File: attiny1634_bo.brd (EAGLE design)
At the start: 49.5 x 22.2 mm, 11 parts, among them J1 AVR_SPI_PRG_6NS, Y1 12MHz

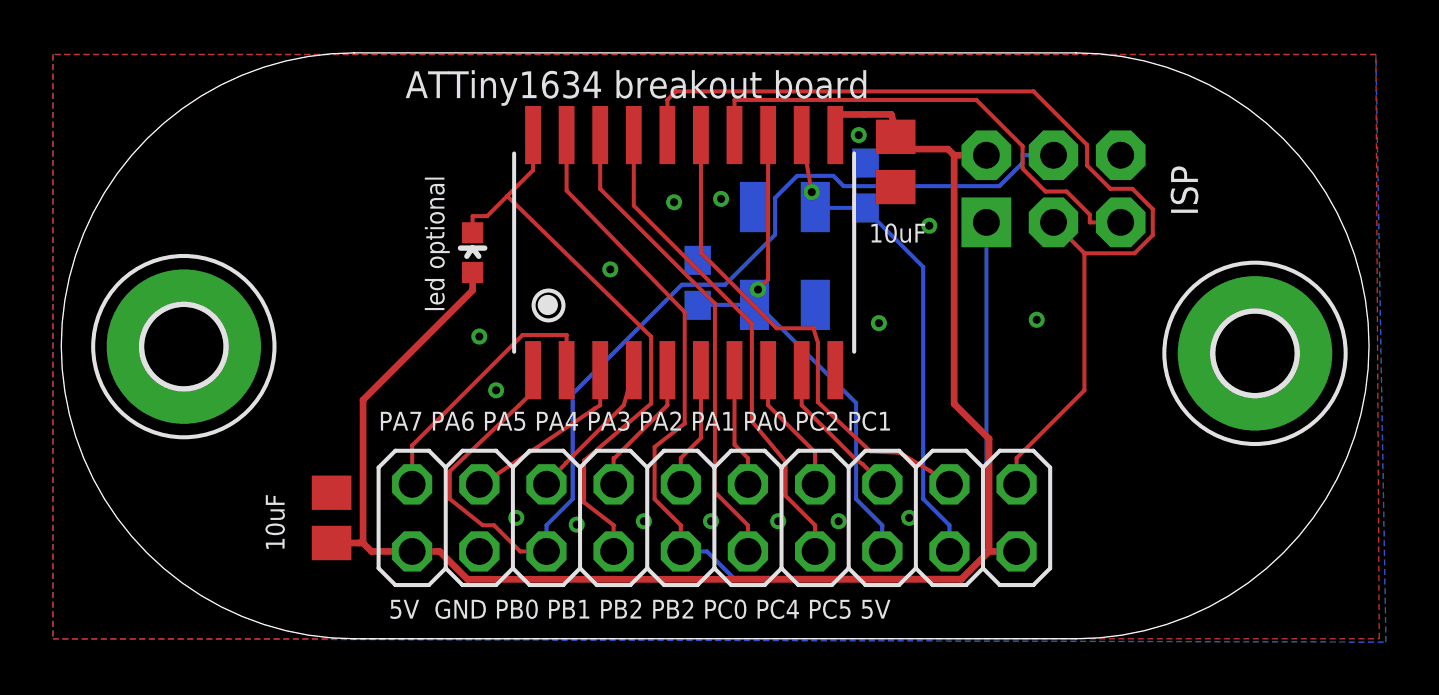
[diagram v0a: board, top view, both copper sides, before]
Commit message: I think it is now good enough
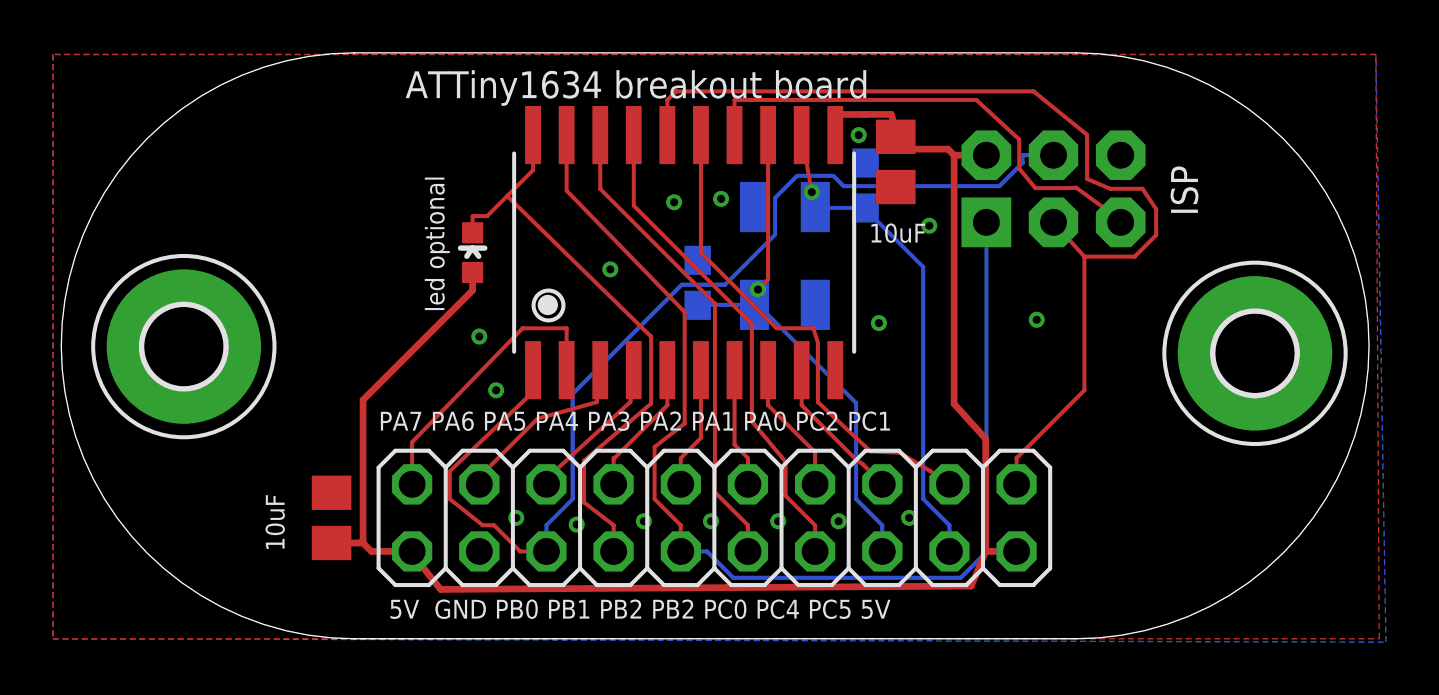
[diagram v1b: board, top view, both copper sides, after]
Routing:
- net PC1/SCL/ADC10: track 37.4 -> 38.1 mm
- net +5V: track 62.5 -> 63.2 mm
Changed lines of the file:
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@@
 <contactref element="U$1" pad="11"/>
 <wire x1="34.0867" y1="18.288" x2="34.0867" y2="8.8837" width="0.254" layer="1"/>
-<wire x1="34.0867" y1="8.8837" x2="35.4075" y2="7.5629" width="0.254" layer="1"/>
-<wire x1="35.4075" y1="7.5629" x2="35.4075" y2="3.302" width="0.254" layer="1"/>
+<wire x1="34.0867" y1="8.8837" x2="35.2805" y2="7.5629" width="0.254" layer="1"/>
+<wire x1="35.2805" y1="7.5629" x2="35.2805" y2="3.302" width="0.254" layer="1"/>
 <wire x1="34.1884" y1="18.288" x2="34.0867" y2="18.288" width="0.254" layer="1"/>
 <wire x1="35.306" y1="18.288" x2="34.1884" y2="18.288" width="0.254" layer="1"/>
@@
 <wire x1="11.5705" y1="3.622" x2="11.7305" y2="3.622" width="0.254" layer="1"/>
 <wire x1="15.875" y1="13.855" x2="15.875" y2="13.1755" width="0.254" layer="1"/>
-<wire x1="13.589" y1="3.302" x2="14.6305" y2="3.302" width="0.254" layer="1"/>
-<wire x1="36.449" y1="3.302" x2="35.4075" y2="3.302" width="0.254" layer="1"/>
-<wire x1="35.4075" y1="3.302" x2="34.3525" y2="2.247" width="0.254" layer="1"/>
-<wire x1="34.3525" y1="2.247" x2="15.6855" y2="2.247" width="0.254" layer="1"/>
-<wire x1="15.6855" y1="2.247" x2="14.6305" y2="3.302" width="0.254" layer="1"/>
+<wire x1="13.589" y1="3.302" x2="13.6145" y2="3.175" width="0.254" layer="1"/>
+<wire x1="36.449" y1="3.302" x2="35.2805" y2="3.302" width="0.254" layer="1"/>
+<wire x1="35.2805" y1="3.302" x2="34.7335" y2="1.993" width="0.254" layer="1"/>
+<wire x1="34.7335" y1="1.993" x2="14.6695" y2="1.866" width="0.254" layer="1"/>
+<wire x1="14.6695" y1="1.866" x2="13.6145" y2="3.175" width="0.254" layer="1"/>
 <wire x1="31.877" y1="18.5193" x2="33.8554" y2="18.5193" width="0.254" layer="1"/>
 <wire x1="33.8554" y1="18.5193" x2="34.0867" y2="18.288" width="0.254" layer="1"/>
@@
 <contactref element="JP1" pad="1"/>
 <wire x1="36.449" y1="5.842" x2="36.449" y2="6.8327" width="0.1524" layer="1"/>
-<wire x1="39.0146" y1="14.5794" x2="37.846" y2="15.748" width="0.1524" layer="1"/>
+<wire x1="39.0146" y1="14.4524" x2="37.846" y2="15.748" width="0.1524" layer="1"/>
 <wire x1="23.241" y1="20.3787" x2="23.5659" y2="20.7036" width="0.1524" layer="1"/>
 <wire x1="23.5659" y1="20.7036" x2="37.0917" y2="20.7036" width="0.1524" layer="1"/>
-<wire x1="37.0917" y1="20.7036" x2="39.116" y2="18.6793" width="0.1524" layer="1"/>
-<wire x1="39.116" y1="18.6793" x2="39.116" y2="17.8979" width="0.1524" layer="1"/>
-<wire x1="39.116" y1="17.8979" x2="39.9959" y2="17.018" width="0.1524" layer="1"/>
-<wire x1="39.9959" y1="17.018" x2="40.8315" y2="17.018" width="0.1524" layer="1"/>
-<wire x1="40.8315" y1="17.018" x2="41.6008" y2="16.2487" width="0.1524" layer="1"/>
-<wire x1="41.6008" y1="16.2487" x2="41.6008" y2="15.265" width="0.1524" layer="1"/>
-<wire x1="41.6008" y1="15.265" x2="40.9152" y2="14.5794" width="0.1524" layer="1"/>
-<wire x1="40.9152" y1="14.5794" x2="39.0146" y2="14.5794" width="0.1524" layer="1"/>
-<wire x1="39.0146" y1="14.5794" x2="39.0146" y2="9.3983" width="0.1524" layer="1"/>
+<wire x1="37.0917" y1="20.7036" x2="39.116" y2="19.0603" width="0.1524" layer="1"/>
+<wire x1="39.116" y1="19.0603" x2="39.116" y2="17.3899" width="0.1524" layer="1"/>
+<wire x1="39.116" y1="17.3899" x2="39.9959" y2="17.018" width="0.1524" layer="1"/>
+<wire x1="39.9959" y1="17.018" x2="41.2125" y2="17.018" width="0.1524" layer="1"/>
+<wire x1="41.2125" y1="17.018" x2="41.7278" y2="16.2487" width="0.1524" layer="1"/>
+<wire x1="41.7278" y1="16.2487" x2="41.7278" y2="15.265" width="0.1524" layer="1"/>
+<wire x1="41.7278" y1="15.265" x2="40.9152" y2="14.4524" width="0.1524" layer="1"/>
+<wire x1="40.9152" y1="14.4524" x2="39.0146" y2="14.4524" width="0.1524" layer="1"/>
+<wire x1="39.0146" y1="14.4524" x2="39.0146" y2="9.3983" width="0.1524" layer="1"/>
 <wire x1="39.0146" y1="9.3983" x2="36.449" y2="6.8327" width="0.1524" layer="1"/>
 <wire x1="23.241" y1="19.05" x2="23.241" y2="20.3787" width="0.1524" layer="1"/>
@@
 <contactref element="U$1" pad="14"/>
 <contactref element="J1" pad="5"/>
-<wire x1="40.386" y1="15.748" x2="39.2175" y2="15.748" width="0.1524" layer="1"/>
+<wire x1="40.386" y1="15.748" x2="39.9795" y2="16.129" width="0.1524" layer="1"/>
 <wire x1="25.781" y1="19.05" x2="25.781" y2="20.3787" width="0.1524" layer="1"/>
 <wire x1="25.781" y1="20.3787" x2="34.9277" y2="20.3787" width="0.1524" layer="1"/>
-<wire x1="34.9277" y1="20.3787" x2="36.6774" y2="18.629" width="0.1524" layer="1"/>
-<wire x1="36.6774" y1="18.629" x2="36.6774" y2="17.7809" width="0.1524" layer="1"/>
-<wire x1="36.6774" y1="17.7809" x2="37.5418" y2="16.9165" width="0.1524" layer="1"/>
-<wire x1="37.5418" y1="16.9165" x2="38.3412" y2="16.9165" width="0.1524" layer="1"/>
-<wire x1="38.3412" y1="16.9165" x2="39.2175" y2="16.0402" width="0.1524" layer="1"/>
-<wire x1="39.2175" y1="16.0402" x2="39.2175" y2="15.748" width="0.1524" layer="1"/>
+<wire x1="34.9277" y1="20.3787" x2="36.5504" y2="18.883" width="0.1524" layer="1"/>
+<wire x1="36.5504" y1="18.883" x2="36.5504" y2="17.7809" width="0.1524" layer="1"/>
+<wire x1="36.5504" y1="17.7809" x2="37.1608" y2="17.0435" width="0.1524" layer="1"/>
+<wire x1="37.1608" y1="17.0435" x2="38.3412" y2="17.0435" width="0.1524" layer="1"/>
+<wire x1="38.3412" y1="17.0435" x2="38.7095" y2="17.0562" width="0.1524" layer="1"/>
+<wire x1="38.7095" y1="17.0562" x2="39.9795" y2="16.129" width="0.1524" layer="1"/>
 </signal>
 <signal name="PC5/XTAL1">
@@
 <contactref element="U$1" pad="4"/>
 <wire x1="18.669" y1="5.842" x2="18.8977" y2="6.096" width="0.1524" layer="1"/>
-<wire x1="21.971" y1="10.16" x2="21.59" y2="8.8313" width="0.1524" layer="1"/>
-<wire x1="21.59" y1="8.8313" x2="19.4057" y2="6.647" width="0.1524" layer="1"/>
-<wire x1="19.4057" y1="6.647" x2="18.8977" y2="6.096" width="0.1524" layer="1"/>
+<wire x1="21.971" y1="10.16" x2="21.844" y2="8.9583" width="0.1524" layer="1"/>
+<wire x1="21.844" y1="8.9583" x2="18.8977" y2="6.266" width="0.1524" layer="1"/>
+<wire x1="18.8977" y1="6.266" x2="18.8977" y2="6.096" width="0.1524" layer="1"/>
 </signal>
 <signal name="PA4">
@@
 <contactref element="JP1" pad="19"/>
 <contactref element="U$1" pad="2"/>
-<wire x1="19.431" y1="10.16" x2="19.431" y2="11.4887" width="0.1524" layer="1"/>
-<wire x1="19.431" y1="11.4887" x2="17.766" y2="11.4887" width="0.1524" layer="1"/>
-<wire x1="17.766" y1="11.4887" x2="13.589" y2="7.3117" width="0.1524" layer="1"/>
-<wire x1="13.589" y1="7.3117" x2="13.589" y2="5.842" width="0.1524" layer="1"/>
+<wire x1="19.431" y1="10.16" x2="19.431" y2="11.7427" width="0.1524" layer="1"/>
+<wire x1="19.431" y1="11.7427" x2="17.766" y2="11.7427" width="0.1524" layer="1"/>
+<wire x1="17.766" y1="11.7427" x2="13.589" y2="7.4387" width="0.1524" layer="1"/>
+<wire x1="13.589" y1="7.4387" x2="13.589" y2="5.842" width="0.1524" layer="1"/>
 </signal>
 <signal name="PA6">
 <contactref element="JP1" pad="17"/>
 <contactref element="U$1" pad="3"/>
-<wire x1="16.129" y1="5.842" x2="16.6117" y2="6.096" width="0.1524" layer="1"/>
-<wire x1="20.701" y1="10.16" x2="20.701" y2="8.8313" width="0.1524" layer="1"/>
-<wire x1="20.701" y1="8.8313" x2="20.49" y2="8.7043" width="0.1524" layer="1"/>
-<wire x1="20.49" y1="8.7043" x2="16.6117" y2="6.096" width="0.1524" layer="1"/>
+<wire x1="16.129" y1="5.842" x2="16.4847" y2="6.477" width="0.1524" layer="1"/>
+<wire x1="20.701" y1="10.16" x2="20.574" y2="8.9487" width="0.1524" layer="1"/>
+<wire x1="20.574" y1="8.9487" x2="18.331" y2="8.3233" width="0.1524" layer="1"/>
+<wire x1="18.331" y1="8.3233" x2="16.4847" y2="6.477" width="0.1524" layer="1"/>
 </signal>
 <signal name="PB3/ADC8/OC1A">
